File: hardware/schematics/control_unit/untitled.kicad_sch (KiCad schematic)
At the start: 10 parts, among them T1 Transformer_1P_1S, U18 LM324

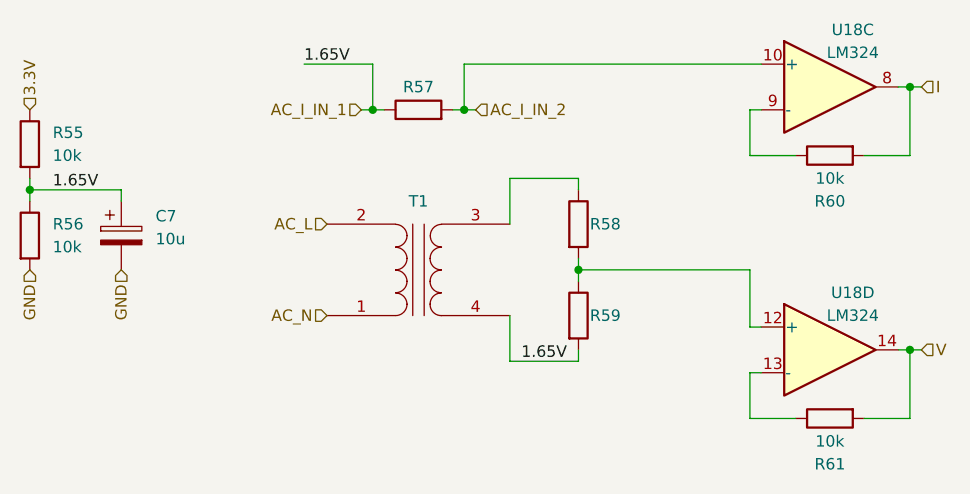
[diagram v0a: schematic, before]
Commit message: !feat
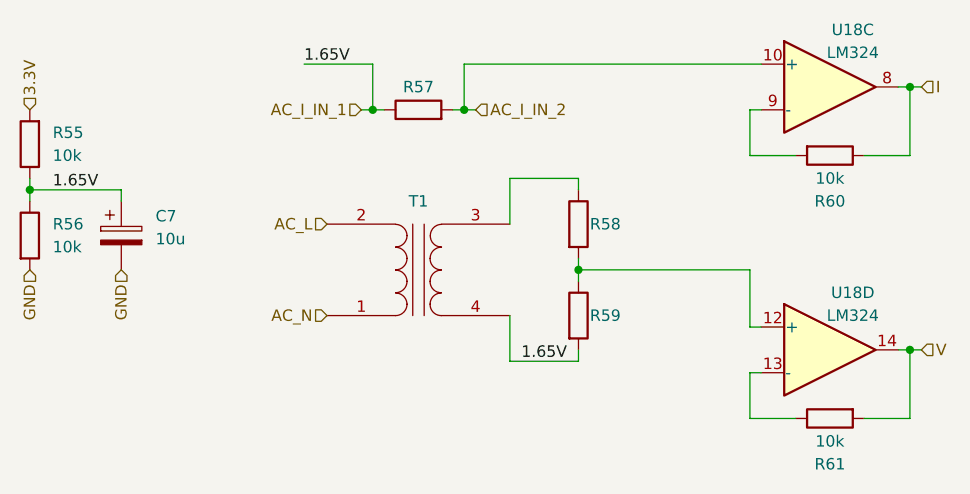
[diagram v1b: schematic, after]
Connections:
- net 3.3V: now also R55.2; no longer R55.1
- net AC_I_IN_1: now also R55.1; no longer R55.2
- net I: now also R60.1; no longer R60.2
- net at U18.9 (-): now also R60.2; no longer R60.1
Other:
- moved on the sheet: R55, R60
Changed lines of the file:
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@@
 	(symbol
 		(lib_id "Device:R")
-		(at 190.5 87.63 90)
-		(mirror x)
+		(at 190.5 87.63 270)
 		(unit 1)
 		(exclude_from_sim no)
@@
 	(symbol
 		(lib_id "Device:R")
-		(at 101.6 86.36 0)
+		(at 101.6 86.36 180)
 		(unit 1)
 		(exclude_from_sim no)
@@
 					(size 1.27 1.27)
 				)
-				(justify left)
+				(justify right)
 			)
 		)
@@
 					(size 1.27 1.27)
 				)
-				(justify left)
-			)
-		)
-		(property "Footprint" "Resistor_THT:R_Axial_DIN0207_L6.3mm_D2.5mm_P7.62mm_Horizontal"
-			(at 99.822 86.36 90)
-			(effects
-				(font
+				(justify right)
+			)
+		)
+		(property "Footprint" "Resistor_THT:R_Axial_DIN0207_L6.3mm_D2.5mm_P7.62mm_Horizontal"
+			(at 103.378 86.36 90)
+			(effects
+				(font
